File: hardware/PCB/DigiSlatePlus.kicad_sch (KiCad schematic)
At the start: 44 parts, among them J1 Serial, J10 IO7, J2 USB_B, J6 Slate, J7 Timecode IN, J8 Timecode OUT, J9 MISO, Q4 2N2222, SW1 RotaryEncoder-SW, SW2 1, SW3 1, SW4 1, SW5 1, SW6 BOOT, U1 ESP32-S3-WROOM-1, U2 DS3231M

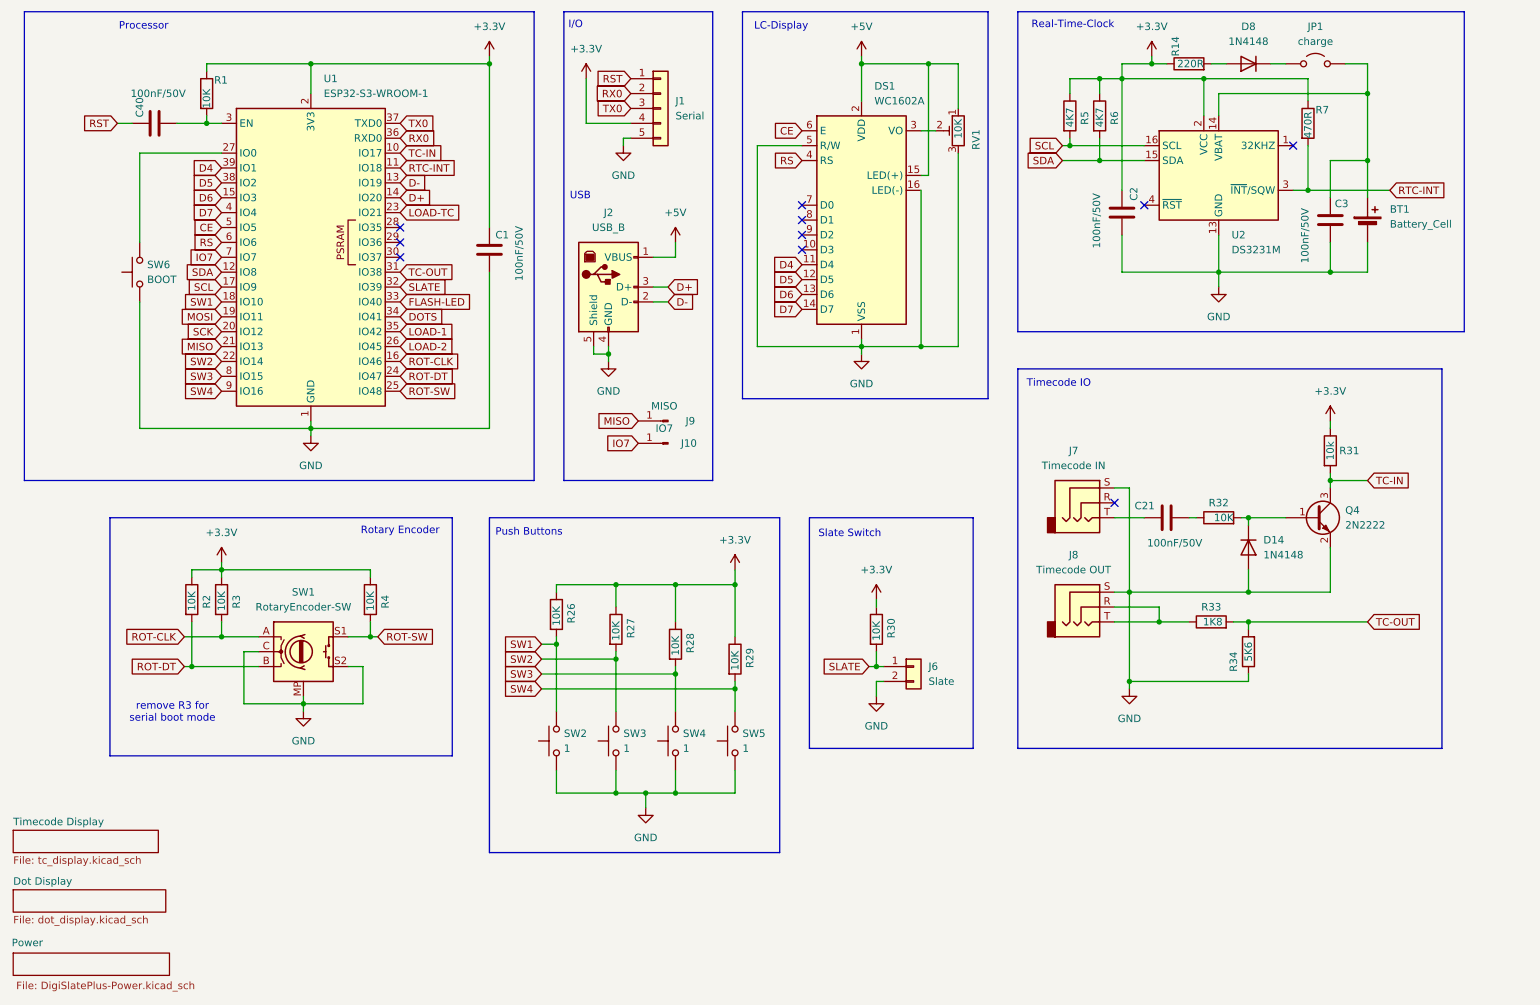
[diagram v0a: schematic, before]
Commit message: Last bug fixes
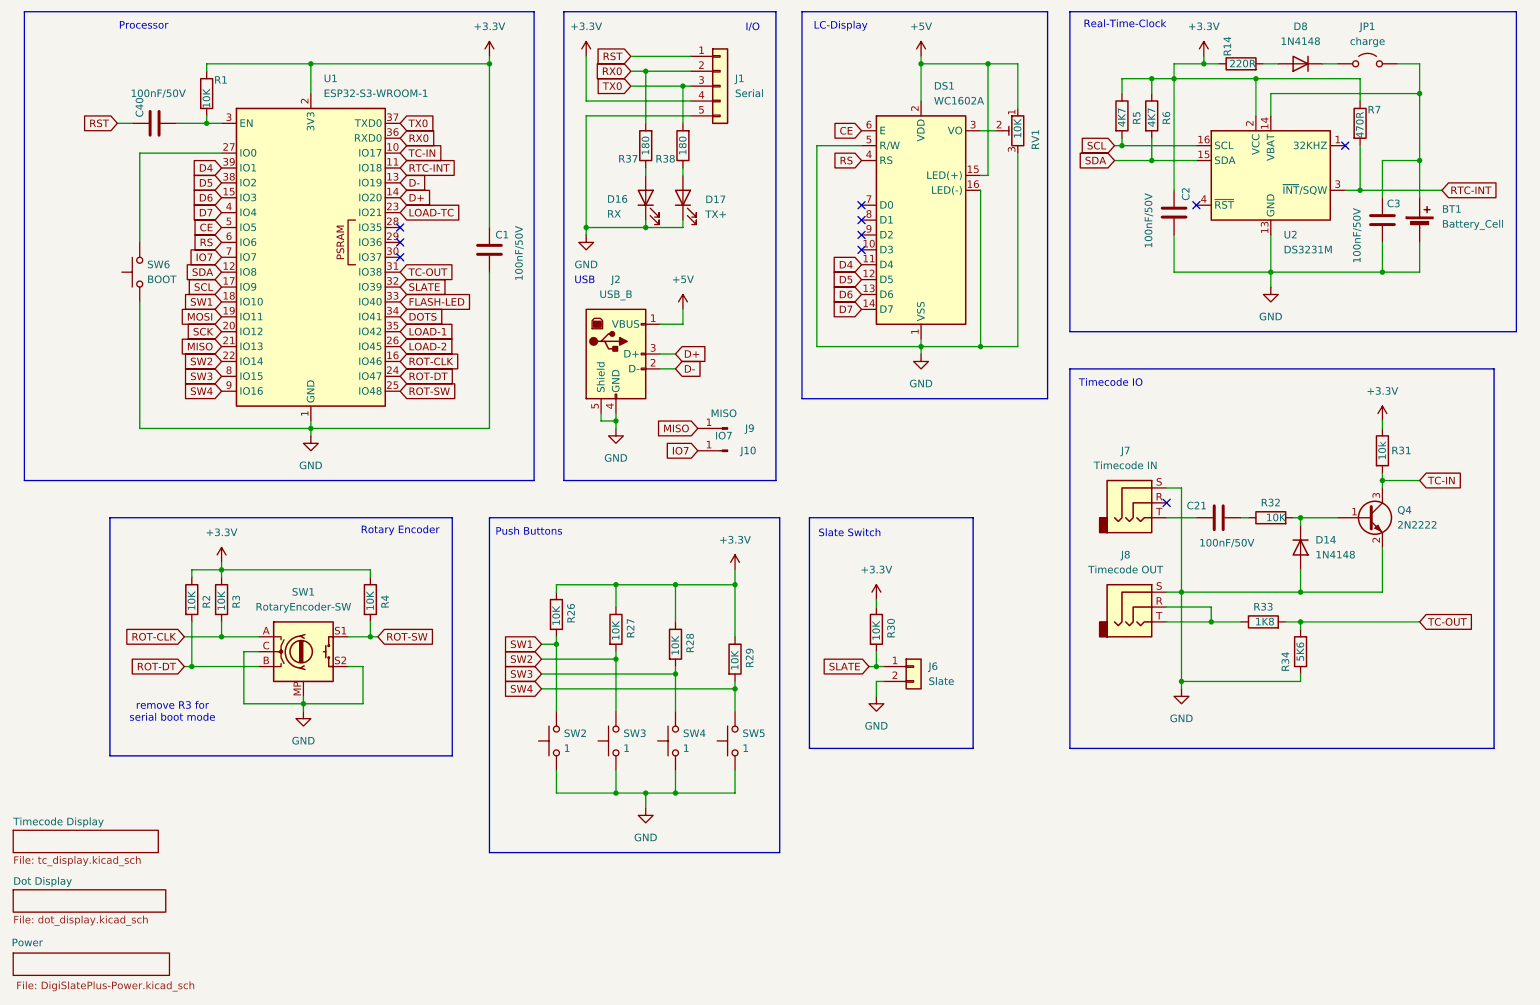
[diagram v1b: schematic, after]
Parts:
- added D16: RX, LED_SMD:LED_0603_1608Metric, symbol Device:LED
- added D17: TX+, LED_SMD:LED_0603_1608Metric, symbol Device:LED
- added R37, R38: 180, Resistor_SMD:R_0805_2012Metric_Pad1.20x1.40mm_HandSolder, symbol Device:R
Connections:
- net GND: now also D16.1 (K), D17.1 (K)
- net RX0: now also R37.2
- net TX0: now also R38.2
- new net: D17.2 (A), R38.1
- new net: D16.2 (A), R37.1
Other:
- moved on the sheet: BT1, C2, C21, C3, D14, D8, DS1, J1, J10, J2, J7, J8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
